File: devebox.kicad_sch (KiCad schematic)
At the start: 27 parts, among them J1 ST-LINK, J2 USB, J3 Right Header, J4 Left Header, SW1 RESET SW, U1 STM32H743VITx, Y1 25MHZ

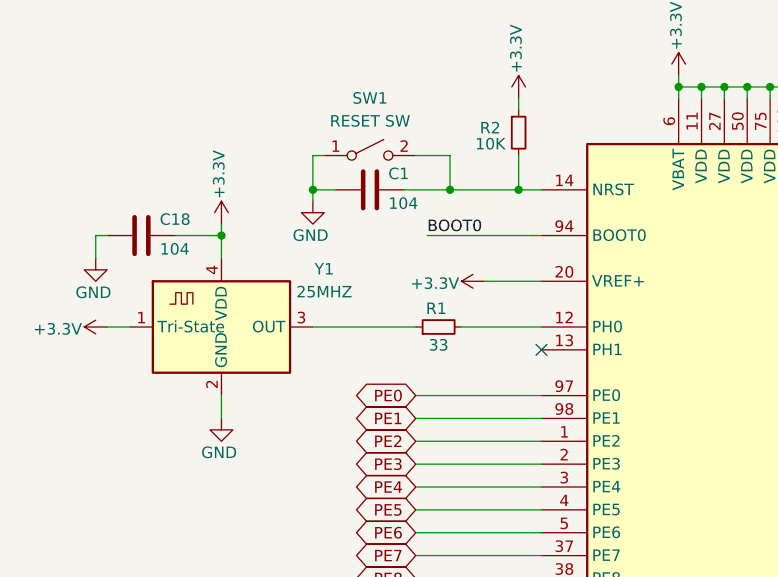
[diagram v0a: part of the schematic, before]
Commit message: snapshot
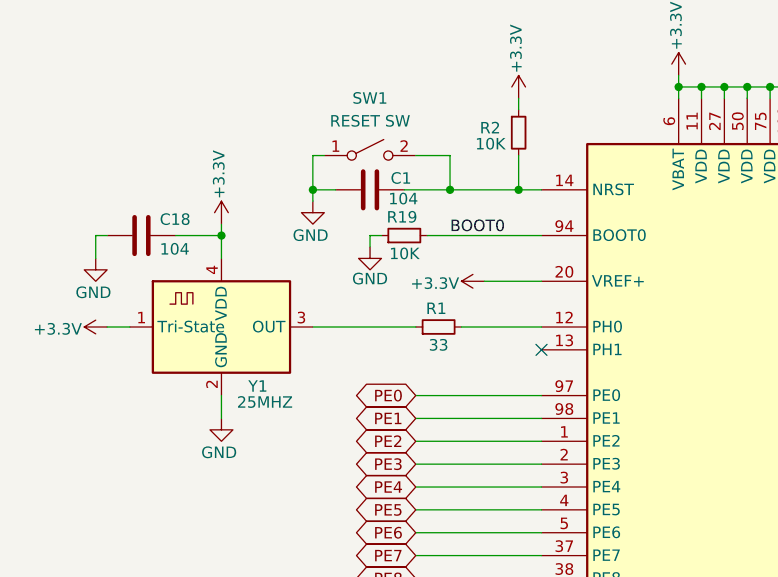
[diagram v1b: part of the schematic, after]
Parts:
- added R19: 10K, Resistor_SMD:R_0805_2012Metric_Pad1.20x1.40mm_HandSolder, symbol LM2676S-3.3_NOPB:R_Small
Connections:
- net BOOT0: now also R19.2
- net GND: now also R19.1
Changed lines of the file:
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@@
 	(wire
 		(pts
+			(xy 55.88 43.18) (xy 55.88 44.45)
+		)
+		(stroke
+			(width 0)
+			(type default)
+		)
+	)
+	(wire
+		(pts
 			(xy 62.23 43.18) (xy 74.93 43.18)
 		)
@@
 	(wire
 		(pts
+			(xy 57.15 43.18) (xy 55.88 43.18)
+		)
+		(stroke
+			(width 0)
+			(type default)
+		)
+	)
+	(wire
+		(pts
 			(xy 60.96 139.7) (xy 74.93 139.7)
 		)
@@
 	)
 	(label "BOOT0"
-		(at 62.23 43.18 0)
+		(at 64.77 43.18 0)
 		(effects
 			(font
@@
 		(dnp no)
 		(property "Reference" "C1"
-			(at 57.912 36.322 90)
+			(at 58.166 36.83 90)
 			(effects
 				(font
@@
 		)
 		(property "Value" "104"
-			(at 57.912 39.624 90)
+			(at 57.912 39.116 90)
 			(effects
 				(font
@@
 		(on_board yes)
 		(dnp no)
-		(fields_autoplaced yes)
 		(property "Reference" "Y1"
-			(at 50.8 46.9198 0)
+			(at 43.434 59.944 0)
 			(effects
 				(font
@@
 		)
 		(property "Value" "25MHZ"
-			(at 50.8 49.4598 0)
+			(at 44.196 61.722 0)
 			(effects
 				(font
@@
 	)
 	(symbol
+		(lib_id "LM2676S-3.3_NOPB:GND")
+		(at 55.88 44.45 0)
+		(unit 1)
+		(exclude_from_sim no)
+		(in_bom yes)
+		(on_board yes)
+		(dnp no)
+		(property "Reference" "#PWR071"
+			(at 55.88 50.8 0)
+			(effects
+				(font
+					(size 1.27 1.27)
+				)
+				(hide yes)
+			)
+		)
+		(property "Value" "GND"
+			(at 55.88 48.006 0)
+			(effects
+				(font
+					(size 1.27 1.27)
+				)
+			)
+		)
+		(property "Footprint" ""
+			(at 55.88 44.45 0)
+			(effects
+				(font
+					(size 1.27 1.27)
+				)
+				(hide yes)
+			)
+		)
+		(property "Datasheet" ""
+			(at 55.88 44.45 0)
+			(effects
+				(font
+					(size 1.27 1.27)
+				)
+				(hide yes)
+			)
+		)
+		(property "Description" "Power symbol creates a global label with name \"GND\" , ground"
+			(at 55.88 44.45 0)
+			(effects
+				(font
+					(size 1.27 1.27)
+				)
+				(hide yes)
+			)
+		)
+		(pin "1"
+		)
+		(instances
+			(project "Main_H743VI"
+				(path "/1c72d2eb-7fb1-49fe-a026-e817f5a7ec43/a876cc3c-46f3-4b62-bd95-490c4538aae6"
+					(reference "#PWR071")
+					(unit 1)
+				)
+			)
+		)
+	)
+	(symbol
 		(lib_id "LM2676S-3.3_NOPB:+3.3V")
 		(at 171.45 121.92 0)
@@
 					(unit 1)
 				)
+			)
+		)
+	)
+	(symbol
+		(lib_id "LM2676S-3.3_NOPB:R_Small")
+		(at 59.69 43.18 90)
+		(unit 1)
+		(exclude_from_sim no)
+		(in_bom yes)
+		(on_board yes)
+		(dnp no)
+		(property "Reference" "R19"
+			(at 59.436 41.148 90)
+			(effects
+				(font
+					(size 1.27 1.27)
+				)
+			)
+		)
+		(property "Value" "10K"
+			(at 59.69 45.212 90)
+			(effects
+				(font
+					(size 1.27 1.27)
+				)
+			)
+		)
+		(property "Footprint" "Resistor_SMD:R_0805_2012Metric_Pad1.20x1.40mm_HandSolder"
+			(at 59.69 43.18 0)
+			(effects
+				(font
+					(size 1.27 1.27)
+				)
+				(hide yes)
+			)
+		)
+		(property "Datasheet" "~"
+			(at 59.69 43.18 0)
+			(effects
+				(font
+					(size 1.27 1.27)
+				)
+				(hide yes)
+			)
+		)
+		(property "Description" "Resistor, small symbol"
+			(at 59.69 43.18 0)
+			(effects
+				(font
+					(size 1.27 1.27)
+				)
+				(hide yes)
+			)
+		)
+		(pin "2"
+		)
+		(pin "1"
+		)
+		(instances
+			(project "Main_H743VI"
+				(path "/1c72d2eb-7fb1-49fe-a026-e817f5a7ec43/a876cc3c-46f3-4b62-bd95-490c4538aae6"
+					(reference "R19")
+					(unit 1)
+				)
